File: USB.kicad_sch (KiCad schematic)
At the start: 14 parts, among them J3 USB_C_Receptacle_USB2.0_16P, U2 CP2102N-Axx-xQFN24

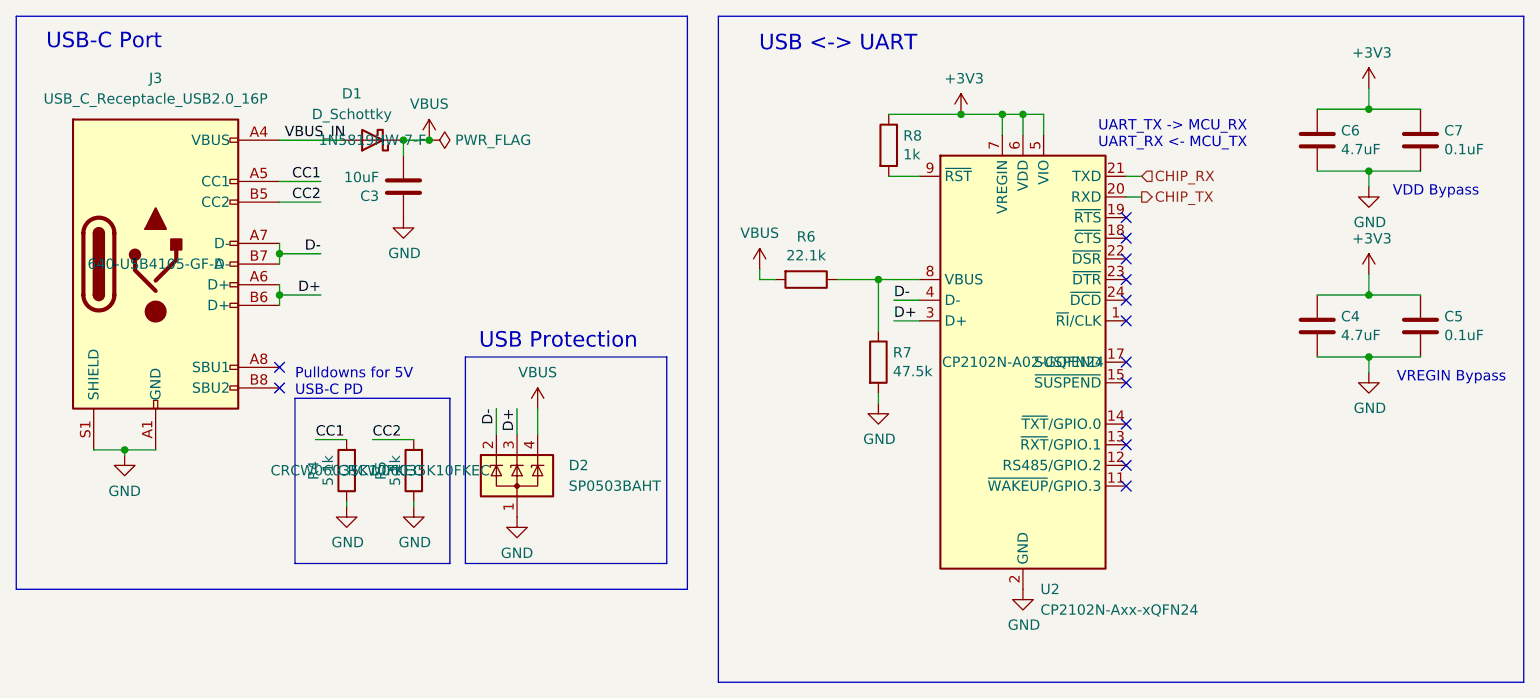
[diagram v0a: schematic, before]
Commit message: updated pins
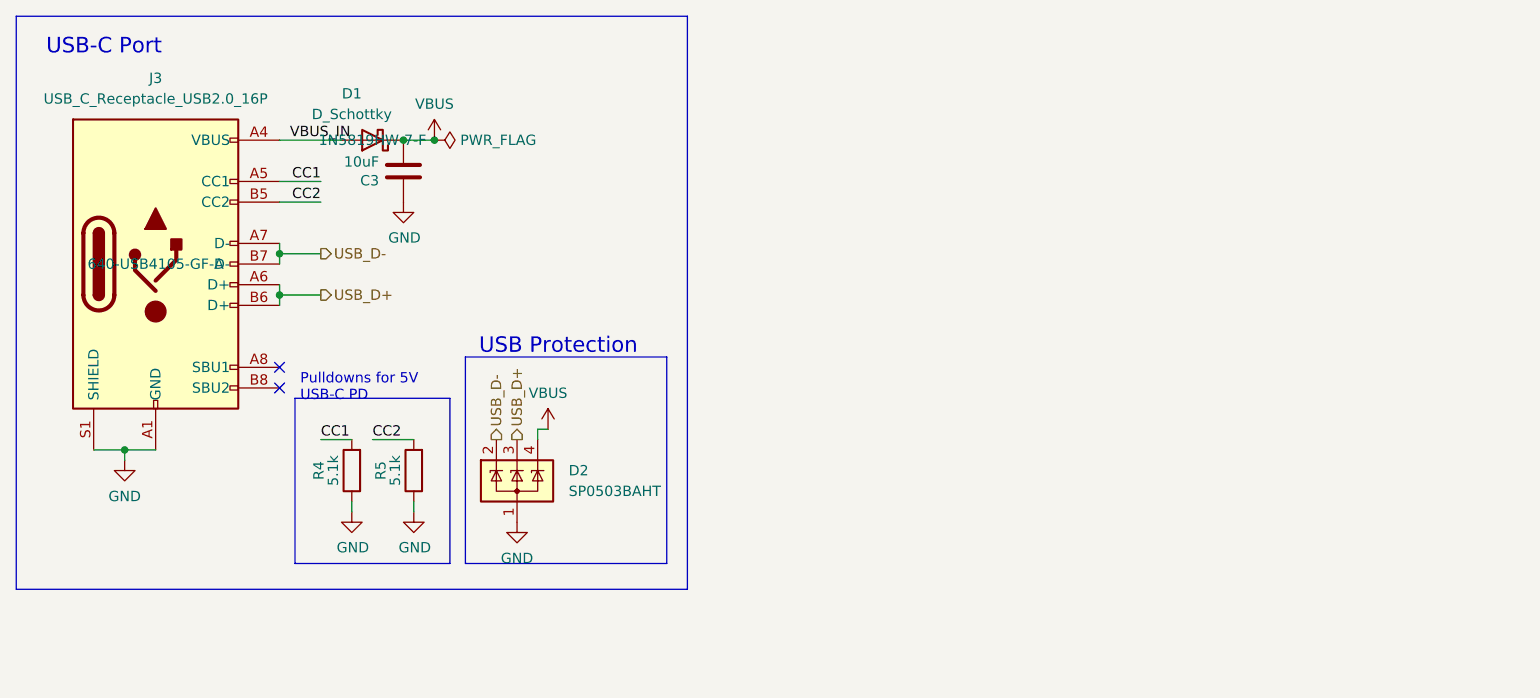
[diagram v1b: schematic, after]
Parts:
- removed C4, C6: 4.7uF, Capacitor_SMD:C_0805_2012Metric, symbol Device:C
- removed C5, C7: 0.1uF, Capacitor_SMD:C_0603_1608Metric_Pad1.08x0.95mm_HandSolder, symbol Device:C
- removed R6: 22.1k, Resistor_SMD:R_0603_1608Metric_Pad0.98x0.95mm_HandSolder, symbol Device:R
- removed R7: 47.5k, Resistor_SMD:R_0603_1608Metric_Pad0.98x0.95mm_HandSolder, symbol Device:R
- removed R8: 1k, Resistor_SMD:R_0603_1608Metric_Pad0.98x0.95mm_HandSolder, symbol Device:R
- removed U2: CP2102N-Axx-xQFN24, UTSVT_ICs:CP2102N-A02-GQFN24, symbol UTSVT-ICs:CP2102N-Axx-xQFN24
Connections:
- net D+ renamed USB_D+
- net D- renamed USB_D-
- no-connect marks 14 -> 2
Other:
- note removed: "UART_TX -> MCU_RX UART_RX <- MCU_TX"
- note removed: "USB <-> UART"
- note removed: "VDD Bypass"
- note removed: "VREGIN Bypass"
- moved on the sheet: C3, D2, R4
